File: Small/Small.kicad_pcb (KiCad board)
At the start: 2 copper layers, 120 x 103.9 mm, 89 parts, among them J1 Conn_Ext_0, J10 Conn_01x03_Female, J11 Conn_01x03_Female, J12 Conn_01x03_Female, J13 Conn_01x03_Female, J14 Conn_01x03_Female, J15 Conn_01x03_Female, J16 Conn_01x03_Female, J17 Conn_01x03_Female, J18 Conn_01x03_Female, J19 Conn_01x03_Female, J2 Conn_Alt_0, J20 Conn_01x03_Female, J21 Conn_01x03_Female, J22 Conn_01x03_Female, J23 Conn_01x03_Female, J24 Conn_01x03_Female, J25 Conn_01x03_Female, J27 SWD_TAG_Connector, J3 Conn_Ext_4, J4 Conn_Alt_4, J5 Conn_Ext_8, J6 Conn_SWD, J7 Conn_Alt_8, J8 Conn_01x03_Female, J9 Conn_01x03_Female, Q1 NMOS, Q2 NMOS, Q3 NMOS, Q4 NMOS, Q5 NMOS, Q6 NMOS, SW1 SW_Push, U1 TLVM23625RDNR, U2 STM32G070KBT6, U3 AP7361C-33E, U4 TXB0102DCU, Y1 Crystal_GND24

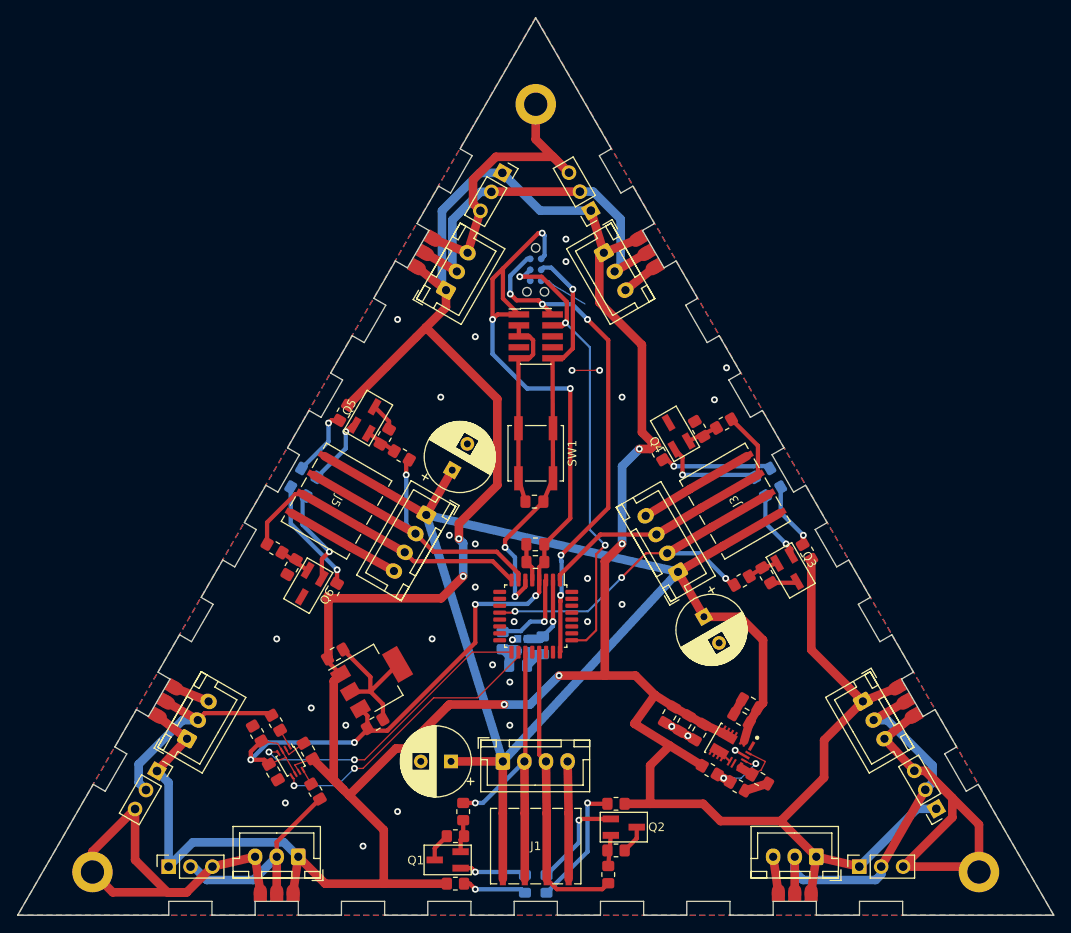
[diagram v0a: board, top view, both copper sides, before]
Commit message: [SMA] Fix many  bug
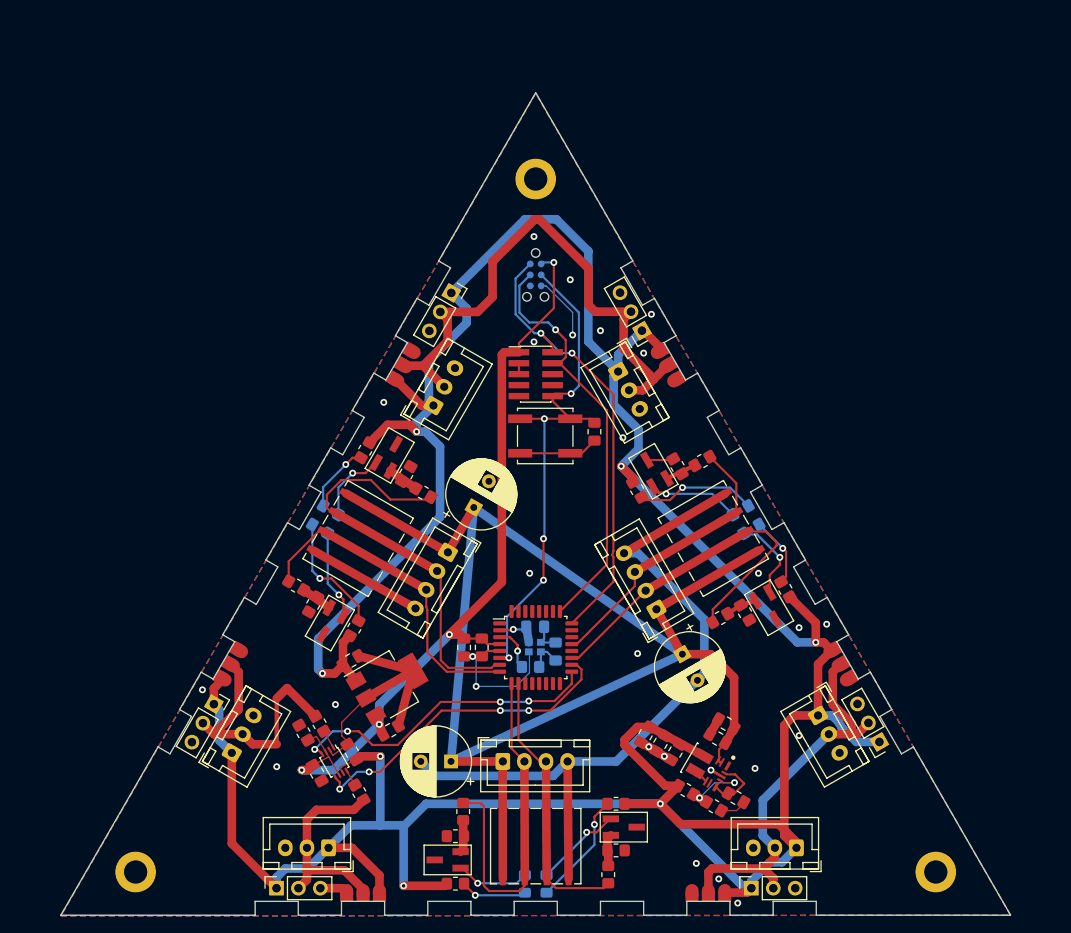
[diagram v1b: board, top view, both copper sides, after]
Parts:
- moved H2 100.3 mm to (28.7, 115.0)
- moved H1 97.7 mm to (121.3, 115.0)
- moved H3 95.3 mm to (75.0, 34.7)
- moved J11 15.1 mm to (87.3, 52.3)
- moved J12 15.1 mm to (65.2, 47.9)
- moved C13 14.5 mm to (66.7, 89.0), turned to -90 degrees
- moved J17 13.9 mm to (84.5, 57.0)
- moved J18 13.4 mm to (63.1, 61.0)
- moved J23 13.2 mm to (91.1, 55.8)
- moved J24 13.2 mm to (58.9, 55.8)
- moved J8 12.7 mm to (45.0, 116.9)
- moved J9 12.7 mm to (100.0, 116.9)
- moved C14 11.7 mm to (68.8, 89.0), turned to -90 degrees
- moved C15 10.7 mm to (81.8, 64.0), turned to -90 degrees
- moved J10 10.2 mm to (114.8, 99.9)
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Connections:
- U2 pad 1: /UART_2_RX -> unconnected-(U2-PB9-Pad1)
- U2 pad 10: unconnected-(U2-PA3-Pad10) -> /UART_1_RX
- U2 pad 12: /UART_2_TX -> unconnected-(U2-PA5-Pad12)
- U2 pad 19: /UART_1_TX -> /UART_2_TX
- U2 pad 21: /UART_1_RX -> /UART_2_RX
- U2 pad 9: unconnected-(U2-PA2-Pad9) -> /UART_1_TX
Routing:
- net GND: track 271.8 -> 184.4 mm, vias 31 -> 27
- net +5V: track 432.8 -> 395.5 mm, vias 6 -> 7
- net +3V3: track 125.1 -> 94.5 mm, vias 7 -> 4
- net Net-(J11-Pin_2): track 43.0 -> 64.4 mm
- net /NRST: track 47.1 -> 61.1 mm, vias 3 -> 5
- net /UART_3_TX: track 37.4 -> 48.0 mm, vias 1 -> 0
- net /SWDIO: track 59.0 -> 53.0 mm, vias 5 -> 2
- net /UART_1_TX: track 35.4 -> 41.0 mm, vias 1 -> 0
- net /OSC_OUT: track 10.2 -> 5.20 mm
- net /SWDCLK: track 53.6 -> 48.7 mm, vias 3 -> 1
- net Net-(J13-Pin_2): track 25.9 -> 30.7 mm
- net /OSC_IN: track 8.93 -> 5.07 mm
- net /UART_2_TX: track 45.2 -> 41.7 mm, vias 3 -> 0
- net VDD: track 168.8 -> 165.4 mm
- net /LED_SIG: track 33.9 -> 37.3 mm, vias 2 -> 4
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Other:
- board size 120 x 103.9 mm -> 110 x 95.3 mm
